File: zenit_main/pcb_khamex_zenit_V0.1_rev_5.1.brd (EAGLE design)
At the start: 146.7 x 215.3 mm, 49 parts, among them IC1 PCA9306JKZ, IC2 SN65HVD230DR, J1 612010235121, J2 52559-2253, J3 686110188622, J4 686110188622, U1 AMS1117-1.8

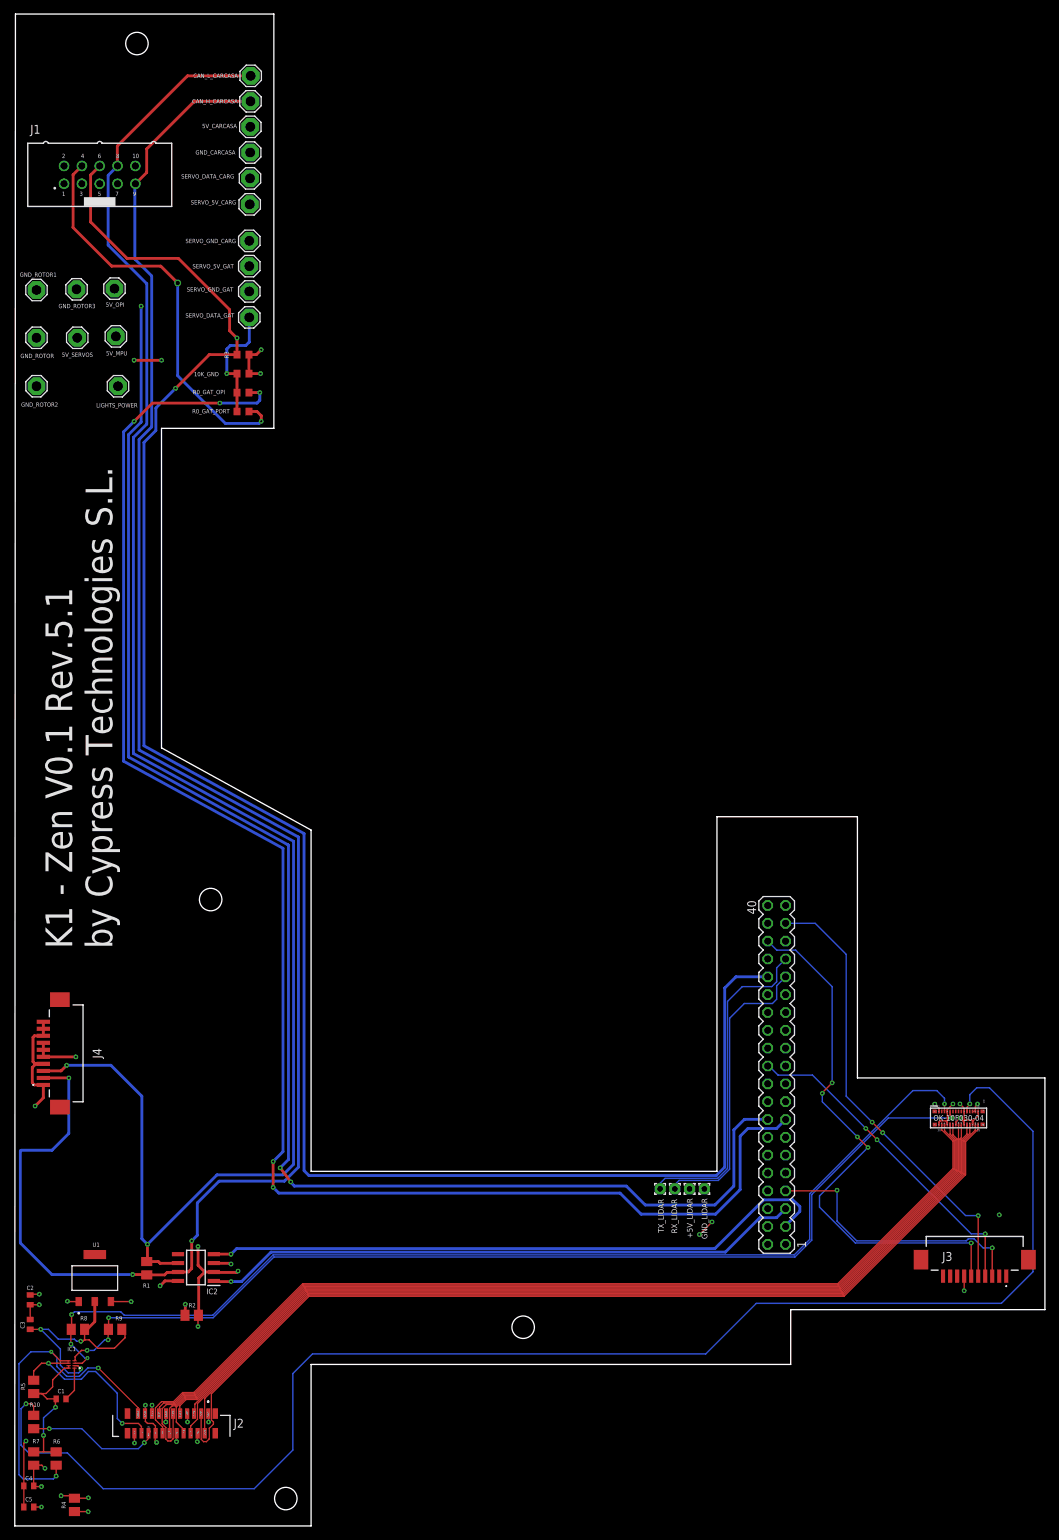
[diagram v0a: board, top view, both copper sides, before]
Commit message: Cambios Juan Carlos
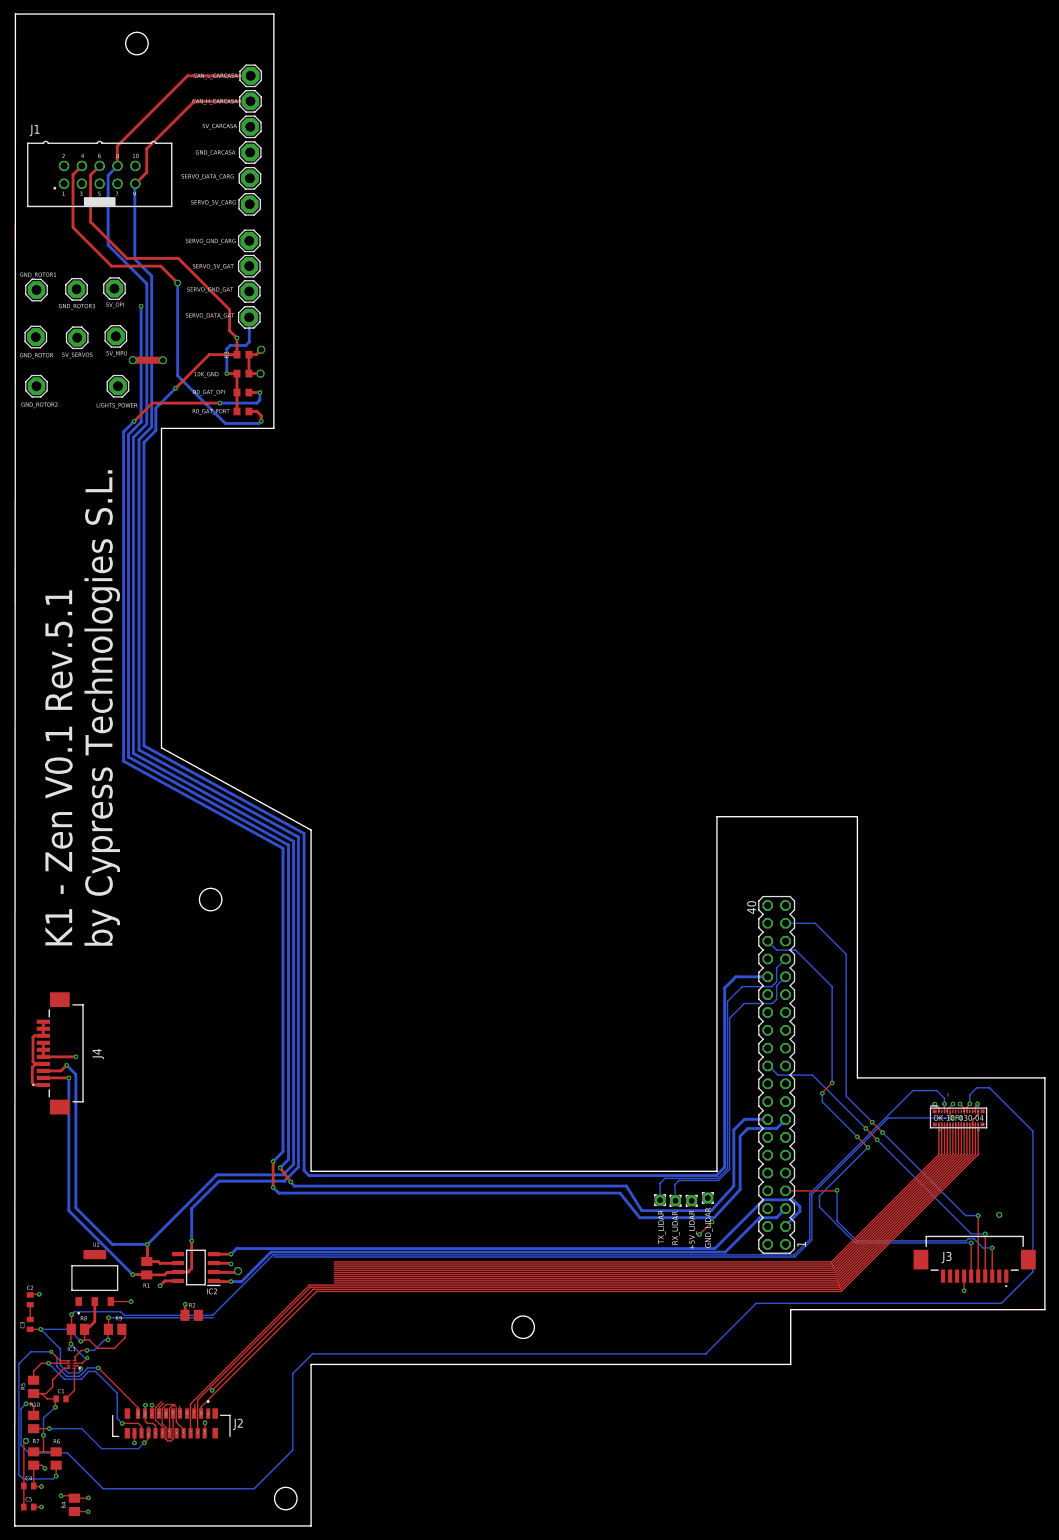
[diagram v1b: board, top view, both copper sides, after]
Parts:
- moved +5V_LIDAR 1.73 mm to (96.4, 46.3)
- moved RX_LIDAR 1.70 mm to (94.1, 46.3)
- moved TX_LIDAR 1.60 mm to (91.9, 46.4)
- moved GND_LIDAR 1.39 mm to (98.7, 46.7)
- moved GND_ROTOR 0.14 mm to (3.00, 169.3)
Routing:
- net GND_PLANE: track 618.6 -> 1036.5 mm, vias 21 -> 10
- net D3N: track 138.7 -> 102.6 mm
- net D3P: track 135.1 -> 99.5 mm
- net D2N: track 143.3 -> 110.3 mm
- net D2P: track 136.5 -> 103.9 mm
- net CLKN: track 136.1 -> 104.5 mm
- net CLKP: track 132.9 -> 102.0 mm
- net D1N: track 131.4 -> 103.3 mm
- net CANH: track 263.9 -> 248.9 mm
- net SDA1: track 146.1 -> 133.9 mm
- net D0P: track 140.1 -> 131.0 mm
- net 5V_MPUS: track 43.6 -> 40.2 mm
- net 5V_OPI: track 255.2 -> 256.9 mm
- net RX_LIDAR: track 42.4 -> 44.1 mm
- net TX_LIDAR: track 47.0 -> 48.6 mm
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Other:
- board text added: "SCL1"
